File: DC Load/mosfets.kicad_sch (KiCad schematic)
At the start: 44 parts, among them Q1 IRFP260, Q2 IRFP260, Q3 IRFP260, Q4 IRFP260, Q5 IRFP260, Q6 IRFP260, Q7 IRFP260, Q8 IRFP260, U1 OPA2182, U2 OPA2182, U3 OPA2182, U4 OPA2182

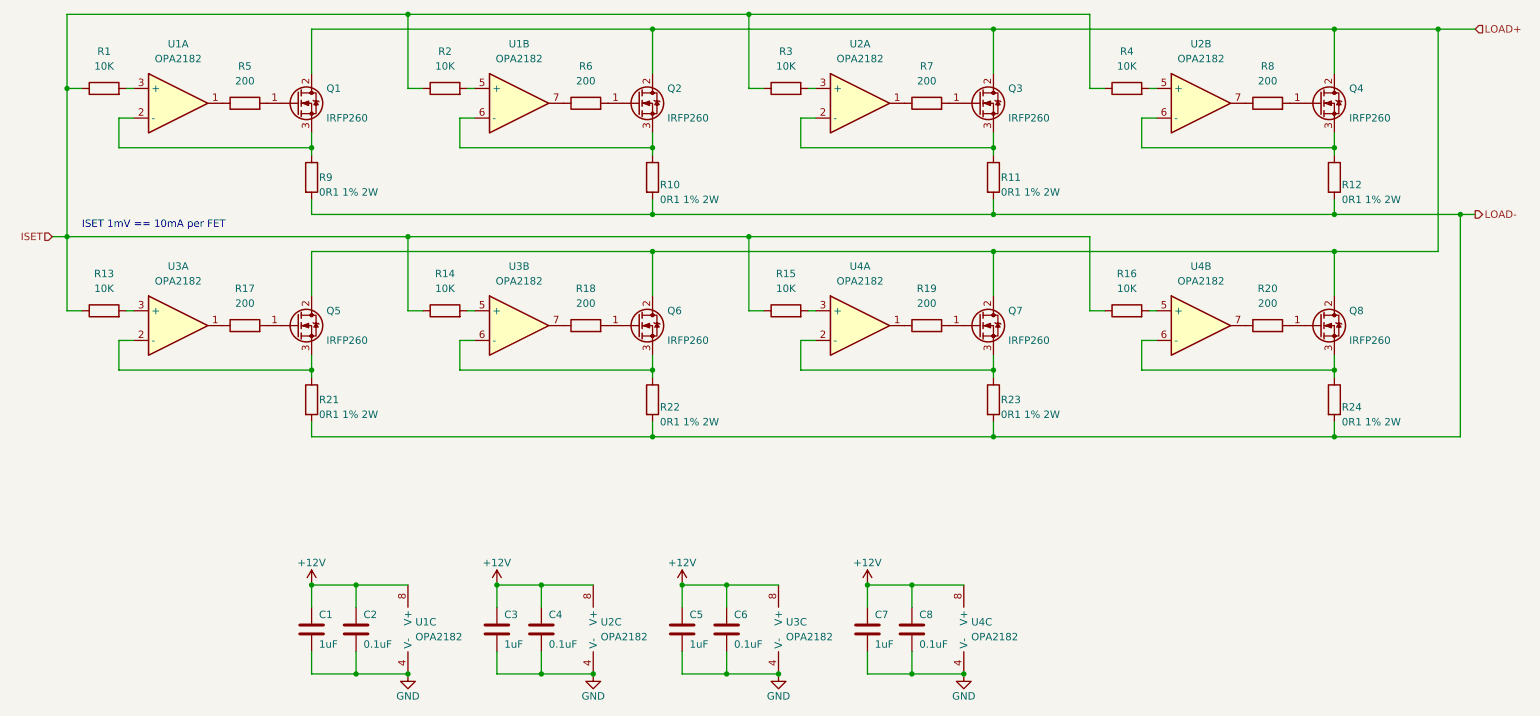
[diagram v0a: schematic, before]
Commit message: Separate sheet for power supply
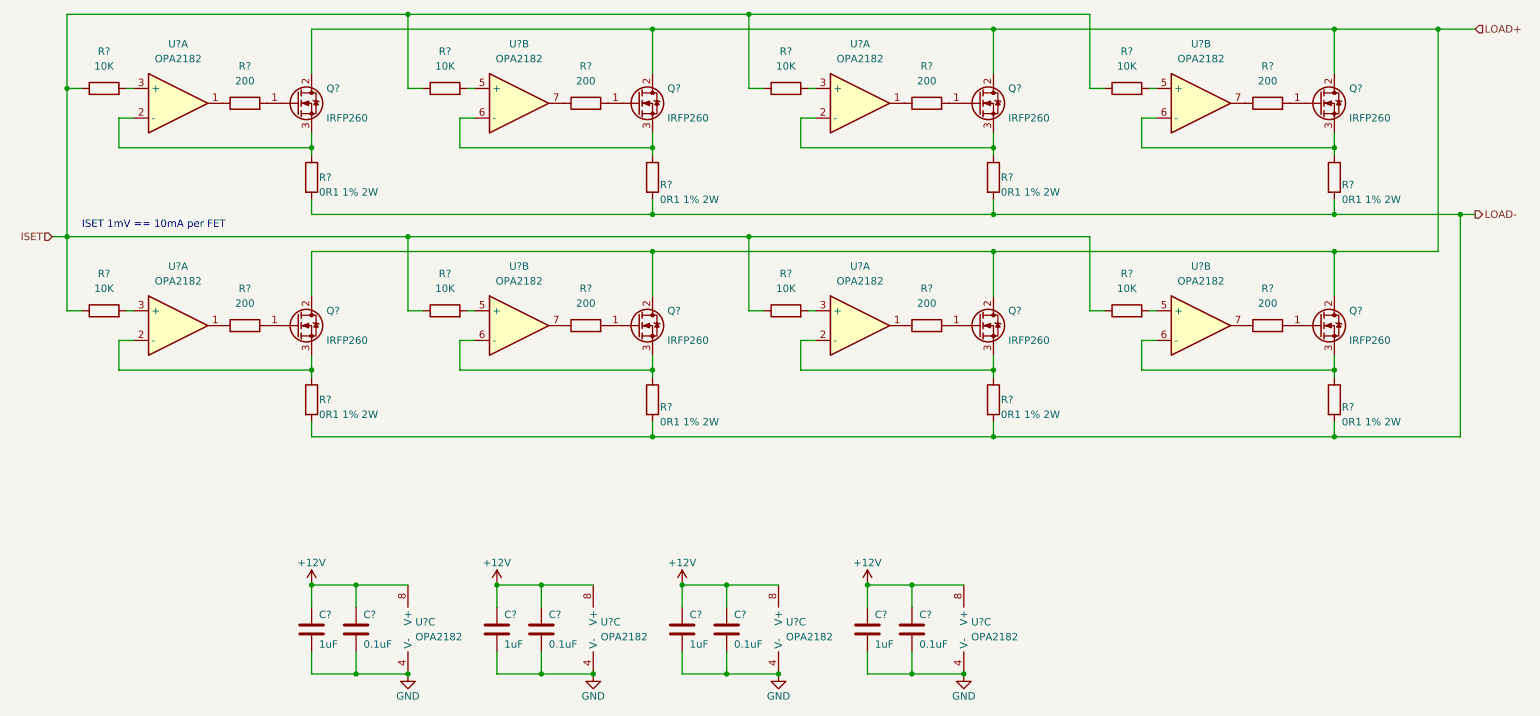
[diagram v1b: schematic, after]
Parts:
- renumbered C1 to C?, C6 to C?, C3 to C?, C8 to C?, C7 to C?, C2 to C?, C5 to C?, C4 to C?, Q4 to Q?, Q5 to Q?, Q8 to Q?, Q2 to Q?, Q7 to Q?, Q1 to Q?, Q3 to Q?, Q6 to Q?, R24 to R?, R11 to R?, R6 to R?, R10 to R?, R13 to R?, R17 to R?, R12 to R?, R23 to R?, R19 to R?, R15 to R?, R20 to R?, R5 to R?, R22 to R?, R16 to R?, R4 to R?, R21 to R?, R2 to R?, R1 to R?, R7 to R?, R3 to R?, R9 to R?, R14 to R?, R8 to R?, R18 to R?, U3 to U?, U1 to U?, U2 to U?, U4 to U?

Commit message: update
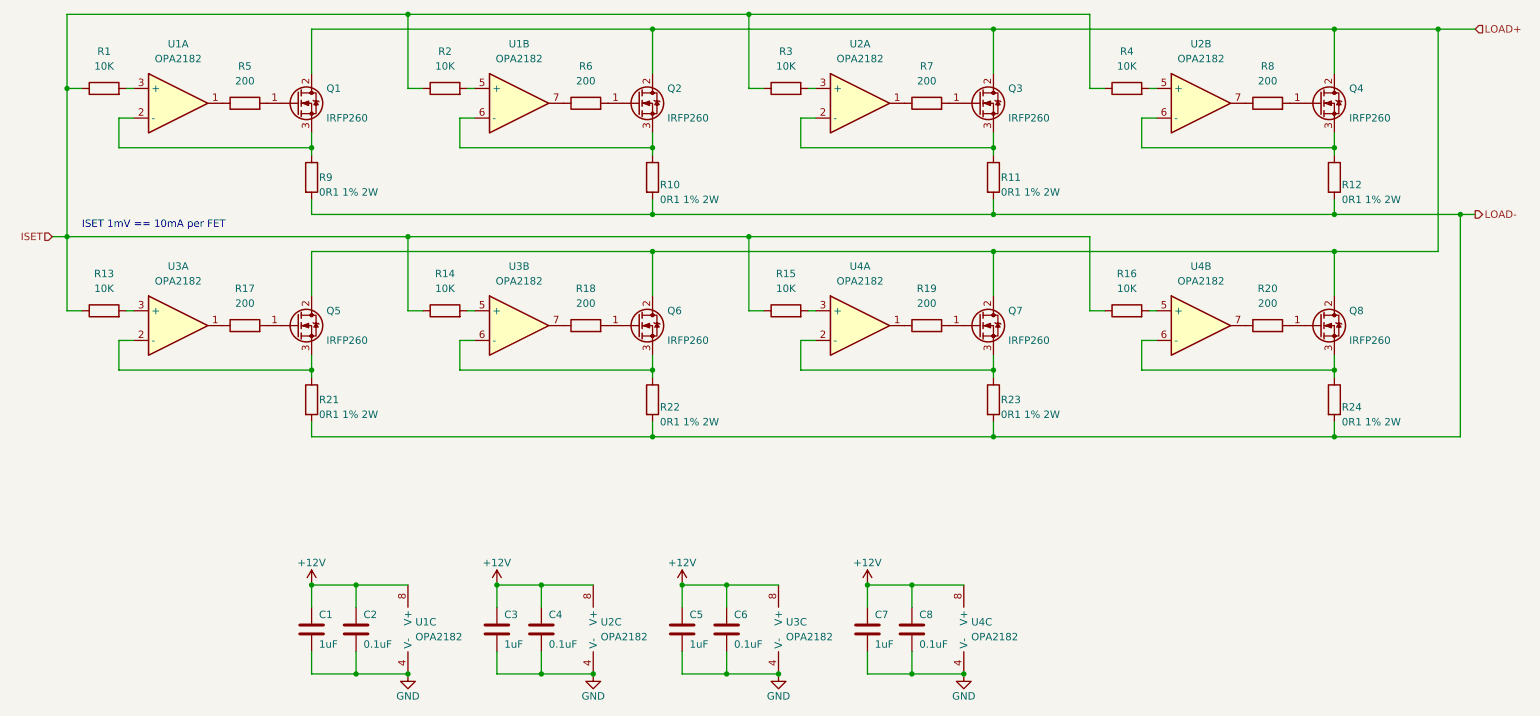
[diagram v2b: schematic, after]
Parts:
- gave numbers to parts that had none: 44
